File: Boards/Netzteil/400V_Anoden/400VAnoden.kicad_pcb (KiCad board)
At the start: 2 copper layers, 160 x 100 mm, 45 parts, among them P1 Drossel, P2 450V_AC, P3 CONN_4, P4 -120V_AC, P5 CONN_4, Q1 2SC2979

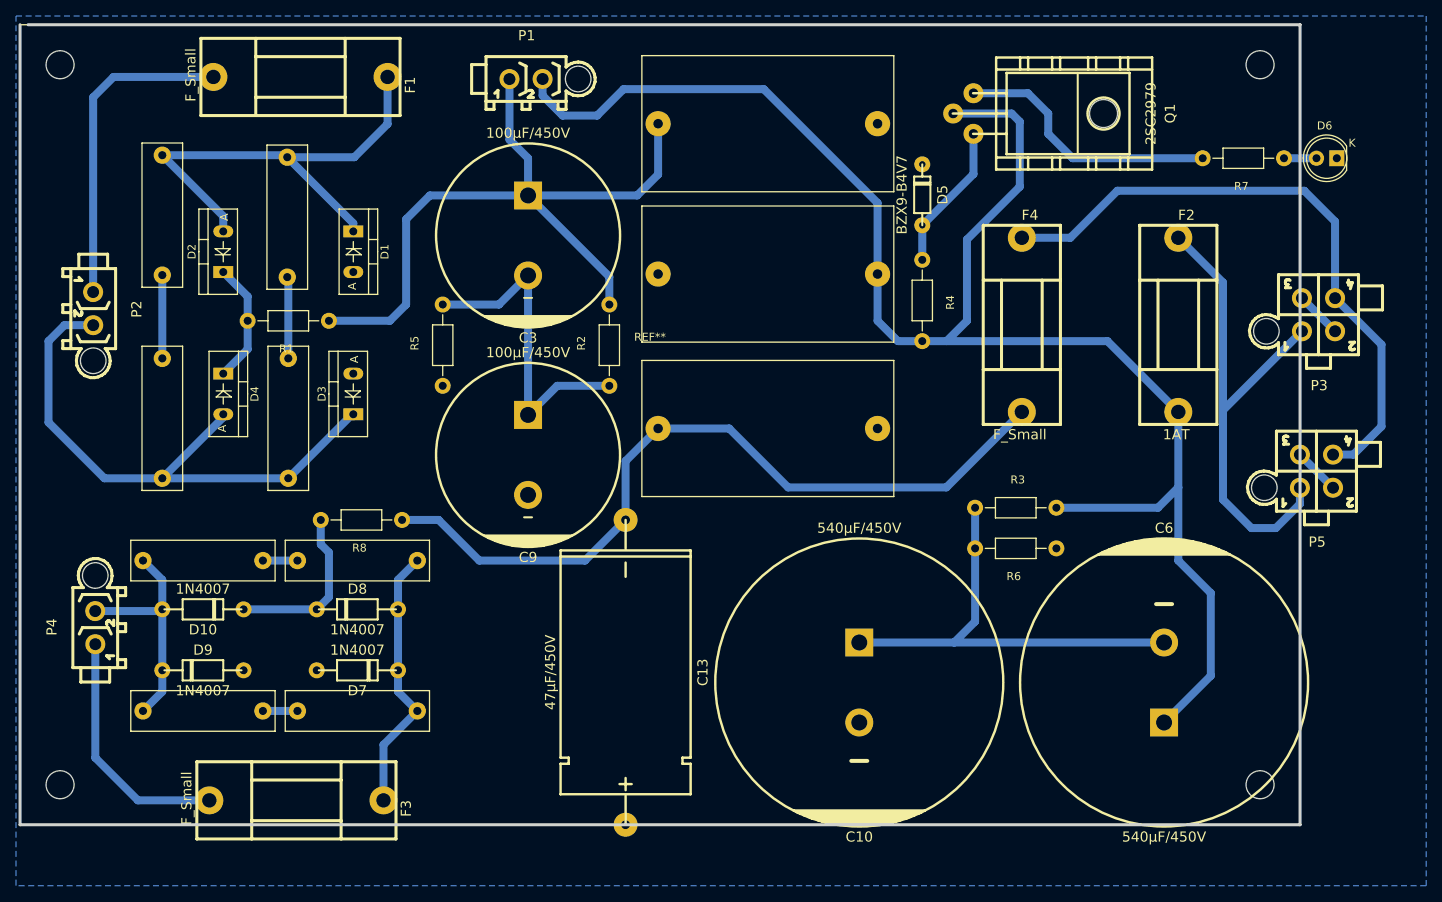
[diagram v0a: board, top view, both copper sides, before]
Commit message: Updated Layout
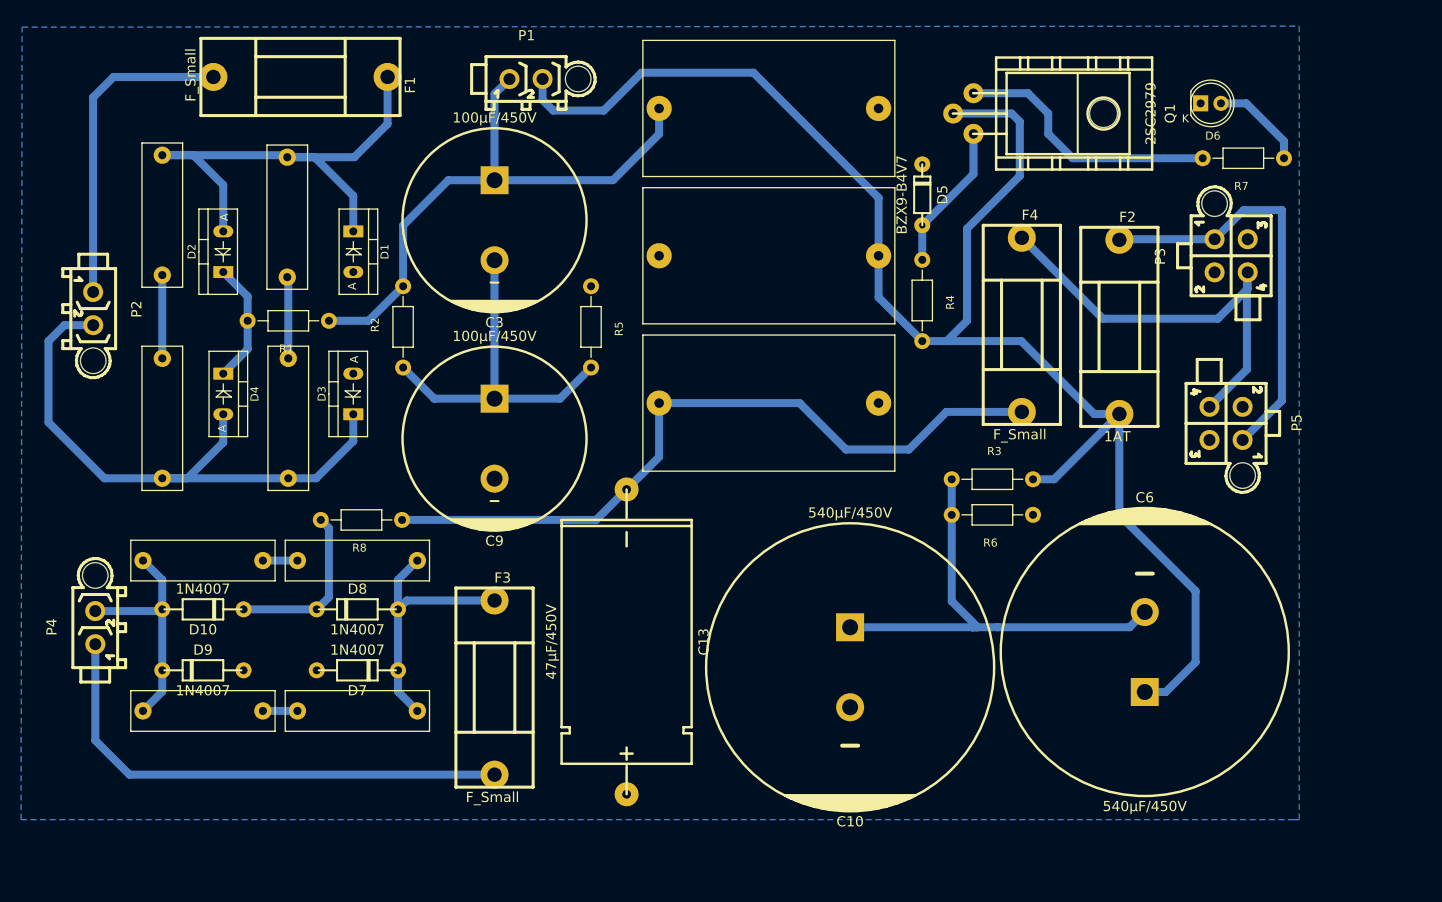
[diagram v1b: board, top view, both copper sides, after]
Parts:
- removed REF**: EuroBoard160mmX100mm_holes, EuroBoard_Outline:EuroBoard160mmX100mm_holes
- moved F3 28.5 mm to (95.9, 109.9), turned to 180 degrees
- moved R2 25.9 mm to (84.5, 64.8)
- moved R5 18.7 mm to (108.0, 64.8), turned to 270 degrees
- moved D6 18.3 mm to (184.2, 36.8), turned to 0 degrees
- moved P3 13.2 mm to (188.0, 55.9), turned to 90 degrees
- moved P5 12.8 mm to (187.3, 76.8), turned to 270 degrees
- moved F2 7.37 mm to (174.0, 64.8)
- moved R6 5.11 mm to (158.1, 88.3)
- moved C9 4.66 mm to (95.9, 78.7)
- moved C3 4.60 mm to (95.9, 51.4)
- moved R3 4.60 mm to (158.1, 83.8)
- moved C6 4.51 mm to (177.2, 105.4)
- moved C13 3.81 mm to (112.4, 104.1)
- moved C14 3.18 mm to (130.2, 74.3)
- moved C5 2.29 mm to (130.2, 55.9)
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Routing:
- net Net-(F3-Pad1): track 30.7 -> 63.7 mm
- net Net-(F4-Pad2): track 78.7 -> 55.1 mm
- net Net-(C3-Pad1): track 94.7 -> 72.6 mm
- net GND: track 12.5 -> 0.00 mm
- net Net-(F2-Pad2): track 63.4 -> 52.6 mm
- net Net-(C5-Pad1): track 208.5 -> 199.2 mm
- net Net-(D6-Pad2): track 4.42 -> 12.0 mm
- net Net-(C13-Pad2): track 97.7 -> 91.8 mm
- net Net-(C1-Pad1): track 62.1 -> 66.4 mm
- net Net-(C7-Pad2): track 73.1 -> 76.9 mm
- net Net-(C10-Pad1): track 56.0 -> 58.3 mm
- net Net-(C3-Pad2): track 42.2 -> 44.0 mm
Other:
- board outline removed

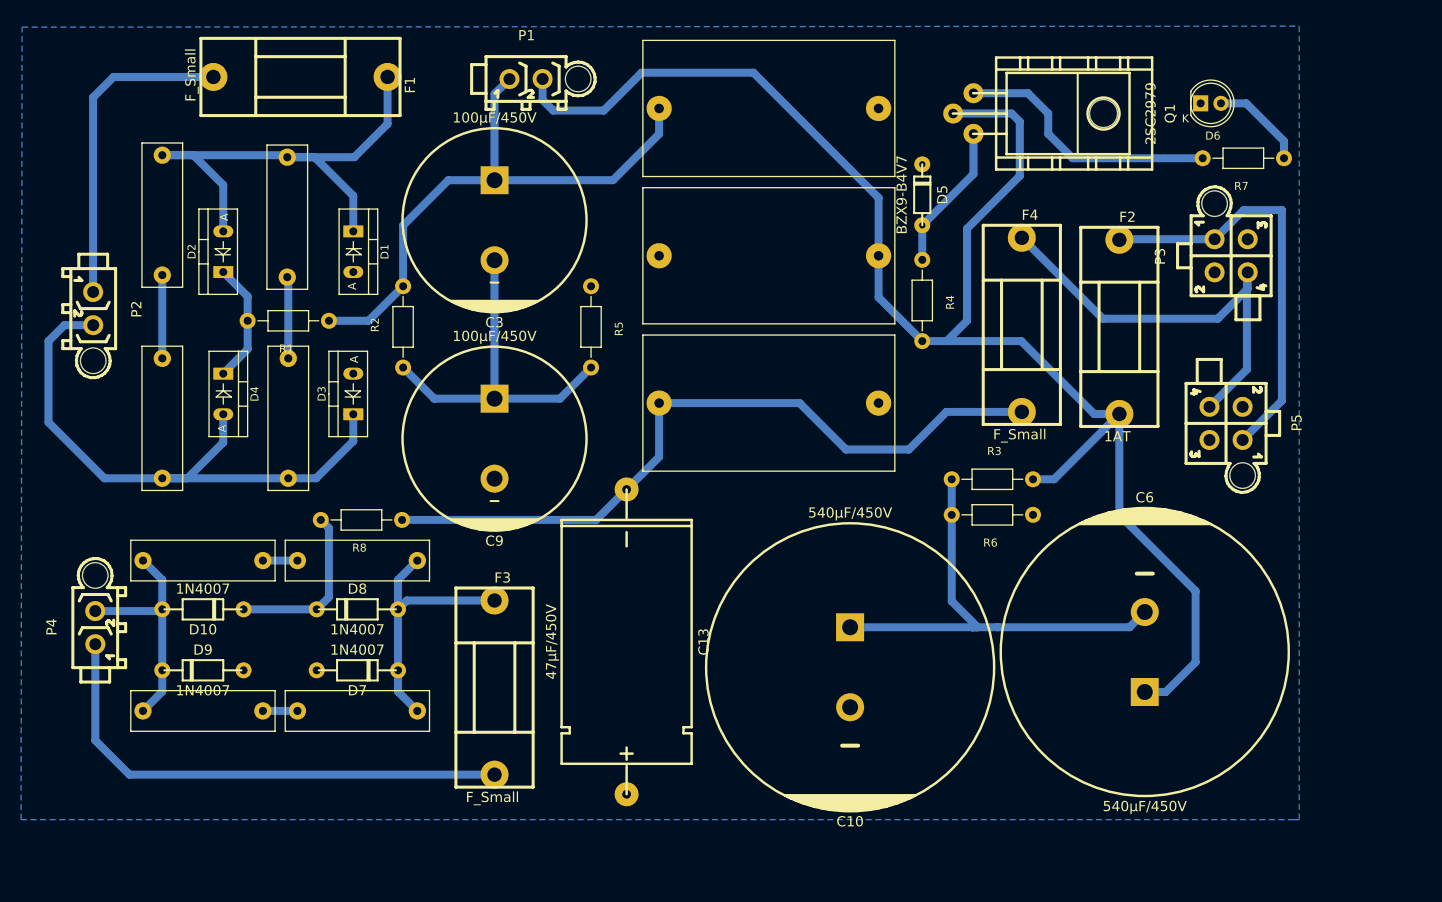
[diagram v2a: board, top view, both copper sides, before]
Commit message: Work in Progress
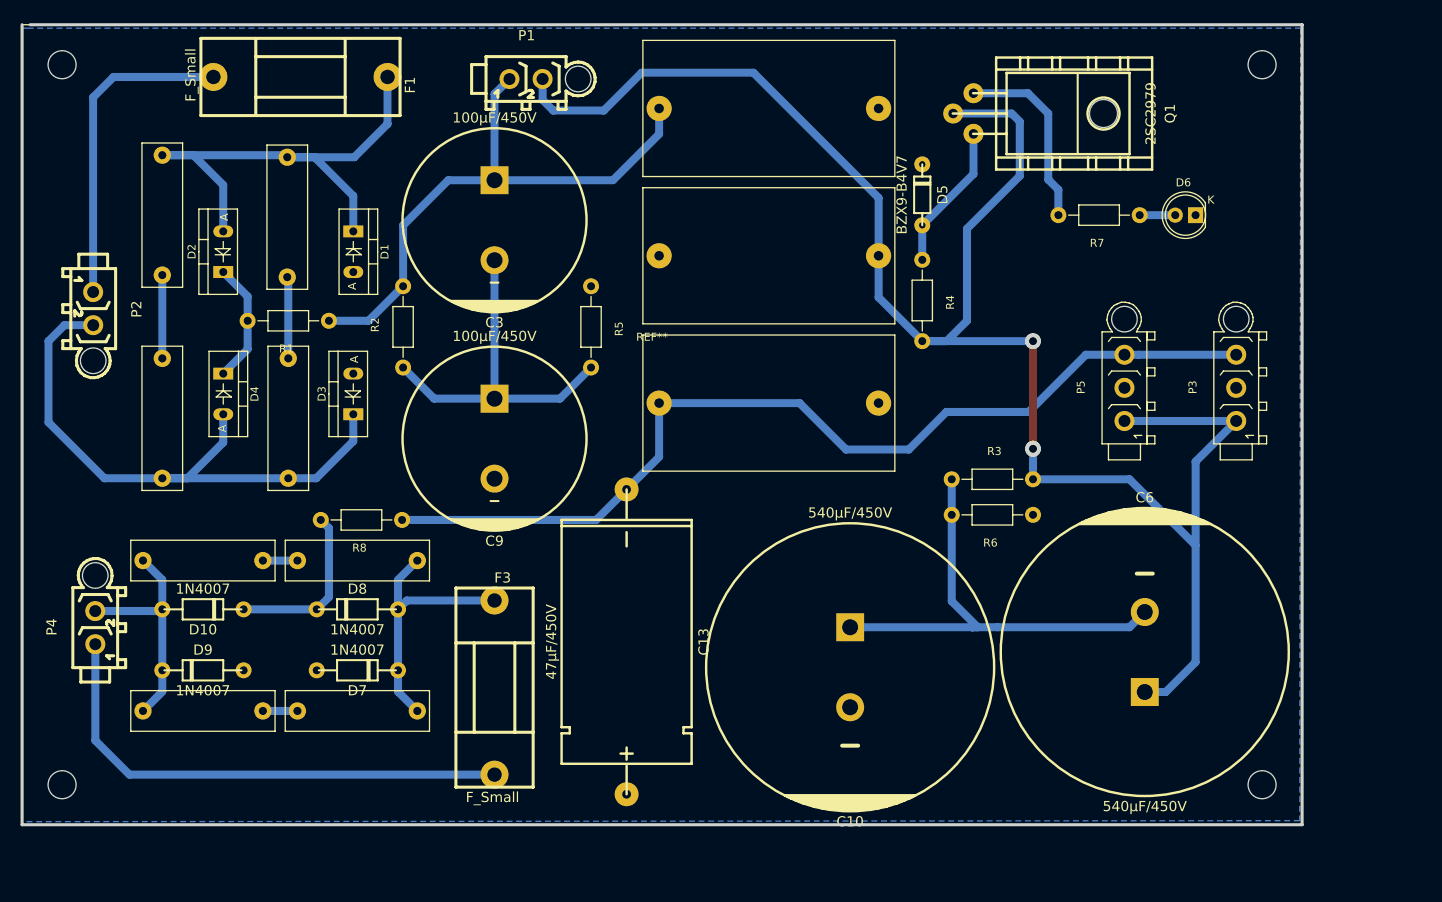
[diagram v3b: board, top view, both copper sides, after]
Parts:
- removed F2: 1AT, w_misc_comp:fuse_holder_CQ-2
- removed F4: F_Small, w_misc_comp:fuse_holder_CQ-2
- added REF**: EuroBoard160mmX100mm_holes, EuroBoard_Outline:EuroBoard160mmX100mm_holes, F.Cu at (36.8, 127.0)
- P2: value 450V_AC -> 320V_AC
- P3, P5: value CONN_4 -> CONN_3; footprint MiniUniversalMate-N-LokSockets_13Aug2012:MiniUniversalMate-N-LokSocket_4PinVertical_13Aug2012 -> Connectors_Mini-Universal:MiniUniversalMate-N-LokSocket_3PinVertical
- P4: value -120V_AC -> 133V_AC
- moved R7 19.4 mm to (171.4, 50.8)
- moved P3 16.5 mm to (188.6, 72.4)
- moved D6 14.0 mm to (183.5, 50.8), turned to 180 degrees
- moved P5 13.5 mm to (174.6, 72.4), turned to 90 degrees
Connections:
- C13 pad 2: Net-(C13-Pad2) -> /-180V_DC
- C14 pad 1: Net-(C13-Pad2) -> /-180V_DC
- C5 pad 1: Net-(C5-Pad1) -> /+450V_DC
- C6 pad 1: Net-(C5-Pad1) -> /+450V_DC
- P1 pad 2: Net-(C5-Pad1) -> /+450V_DC
- P3 pad 1: Net-(F2-Pad2) -> /+450V_DC
- P3 pad 3: GND -> /-180V_DC
- P5 pad 1: Net-(F2-Pad2) -> /+450V_DC
- P5 pad 3: GND -> /-180V_DC
- Q1 pad 2: Net-(C5-Pad1) -> /+450V_DC
- R3 pad 2: Net-(C5-Pad1) -> /+450V_DC
- R4 pad 2: Net-(C5-Pad1) -> /+450V_DC
- R8 pad 1: Net-(C13-Pad2) -> /-180V_DC
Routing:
- net /+450V_DC: track 0.00 -> 225.8 mm, vias 0 -> 2
- net Net-(C5-Pad1): track 199.2 -> 0.00 mm
- net /-180V_DC: track 0.00 -> 121.6 mm
- net Net-(C13-Pad2): track 91.8 -> 0.00 mm
- net Net-(F4-Pad2): track 55.1 -> 0.00 mm
- net Net-(F2-Pad2): track 52.6 -> 0.00 mm
- net Net-(Q1-Pad3): track 33.5 -> 23.6 mm
- net Net-(D6-Pad2): track 12.0 -> 4.44 mm
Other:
- board outline added: 160 x 100 mm
